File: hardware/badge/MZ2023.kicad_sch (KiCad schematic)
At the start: 30 parts, among them J1 Conn_01x04, J2 Conn_01x04, J3 Conn_01x04, J4 Conn_01x04, J5 Conn_01x08_Female, J6 Conn_01x02_Male, J7 Conn_01x07_Female, Q2 DMG2301L, SW1 SW_Push, SW2 SW_Push, SW3 SW_Push, SW4 SW_Push_SPDT, U1 Pico, U3 MCP73831-2-OT

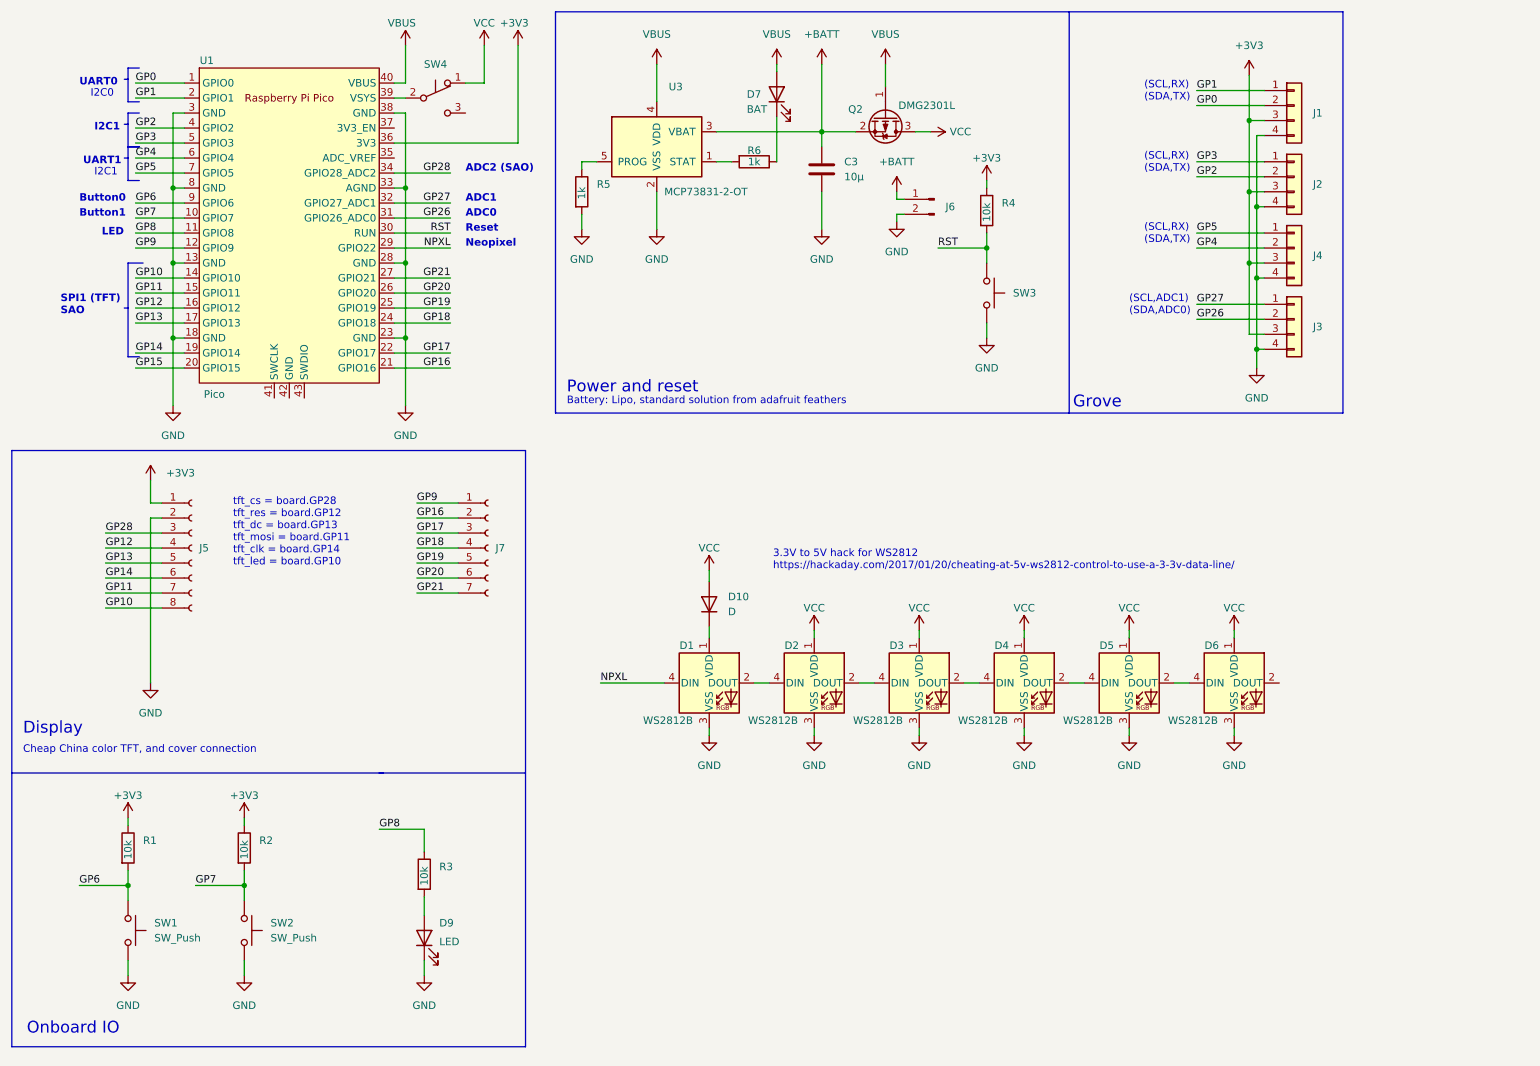
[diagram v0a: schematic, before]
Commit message: WIP
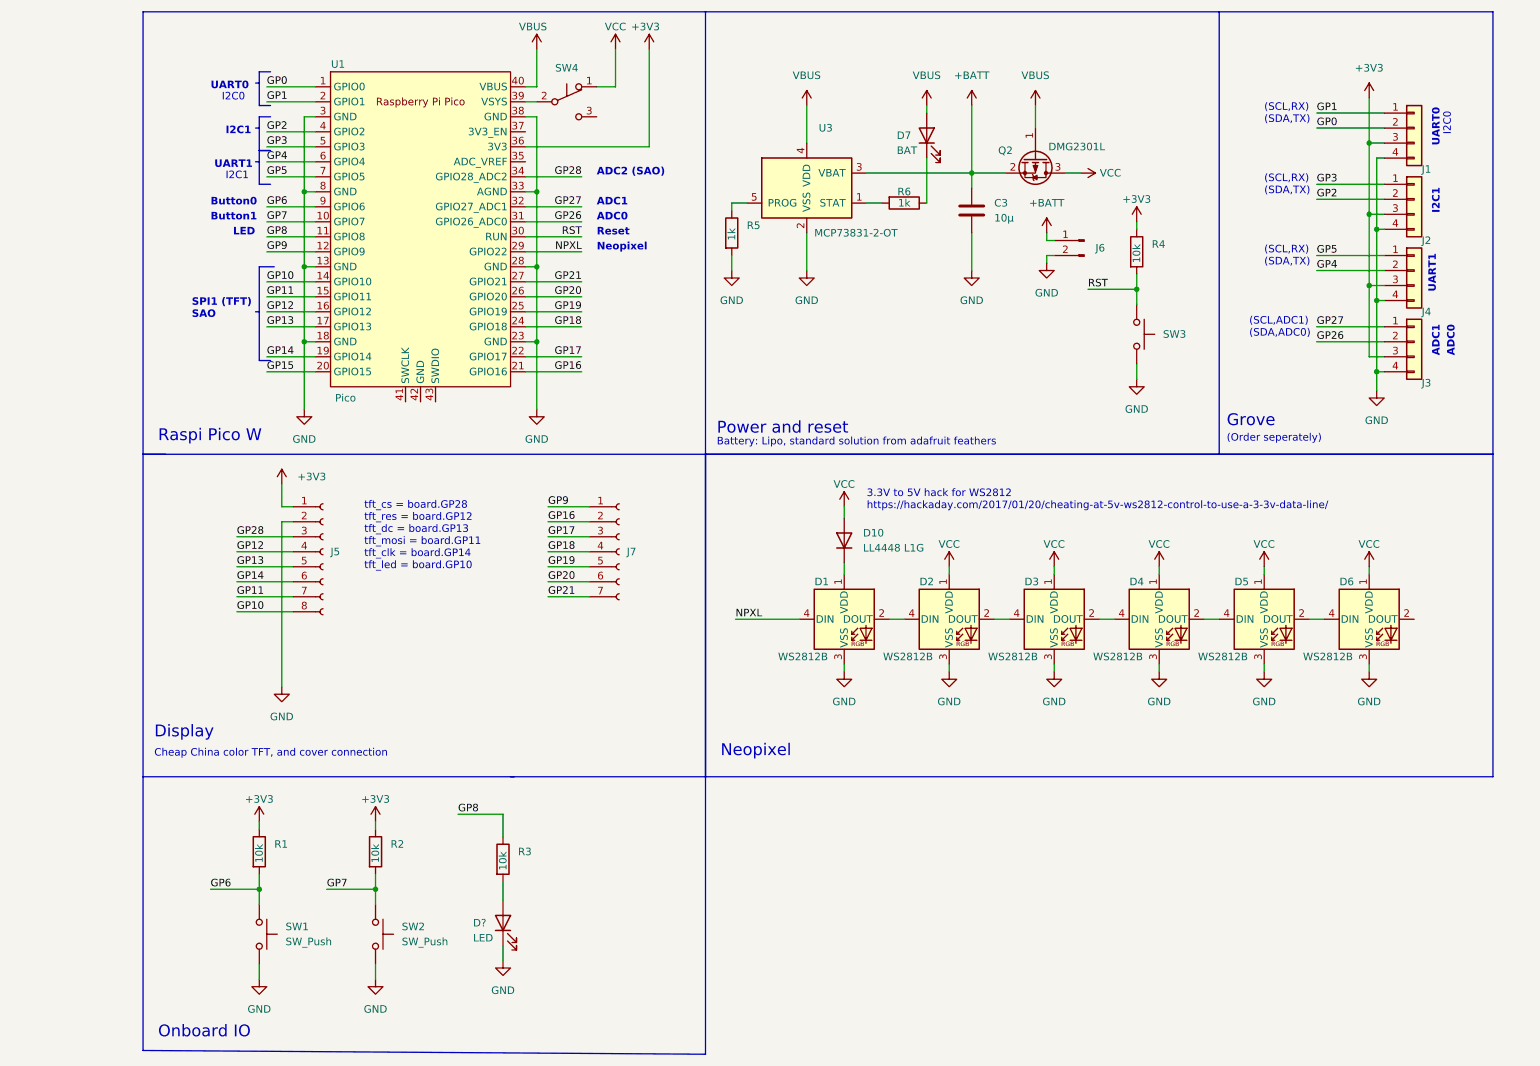
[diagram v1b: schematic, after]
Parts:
- removed D9: LED, LED_SMD:LED_1206_3216Metric_ReverseMount_Hole1.8x2.4mm, symbol Device:LED
- added D?: LED, LED_SMD:LED_0603_1608Metric_Pad1.05x0.95mm_HandSolder, symbol Device:LED
- D1, D2, D3, D4, D5, D6: Digikey (none) -> 1568-COM-16347CT-ND; LCSC (none) -> C114586
- D10: value D -> LL4448 L1G; Digikey (none) -> LL4448L1GCT-ND; LCSC (none) -> C183025; Mouser (none) -> 78-LL4154
- J6: Digikey (none) -> 455-1719-ND; LCSC (none) -> C157932
- Q2: Digitec (none) -> DMG2301L-7DICT-ND; LCSC (none) -> C102619; Mouser (none) -> 621-DMG2301L-7
- SW1, SW2, SW3: Digikey (none) -> CKN10244CT-ND; LCSC (none) -> C269272; Mouser (none) -> 611-KMR221NGLFS
- SW4: Digikey (none) -> CKN9559-ND; LCSC (none) -> C226259; Mouser (none) -> 611-OS102011MA1QN1
- U3: Digikey (none) -> MCP73831T-2ACI/OT; LCSC (none) -> C424093; Mouser (none) -> 579-MCP73831T-2ACIOT
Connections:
- net GND: now also D?.1 (K)
- net at R3.2: now also D?.2 (A)
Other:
- note added: "(Order seperately)"
- note added: "Raspi Pico W"
- company: (none) -> Make Zürich
- title: (none) -> MZ 2023 badge
- moved on the sheet: C3, D1, D10, D2, D3, D4, D5, D6, D7, J1, J2, J3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
